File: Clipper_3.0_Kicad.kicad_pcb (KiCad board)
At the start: 2 copper layers, 19 parts, among them J10 Conn_01x19_Socket, J11 Screw_Terminal_01x02, J12 Conn_01x01_Socket, J13 Conn_01x01_Socket, J14 Conn_01x01_Socket, J15 Conn_01x01_Socket, J4 Conn_01x08_Socket, J5 Conn_01x08_Socket, J6 Conn_01x08_Socket, J9 Conn_01x19_Socket, U1 ESP32-DevKitC, U2 TB6612FNG_MODULE, U3 GY-521 MODULE, U4 DC/DC MINI-360

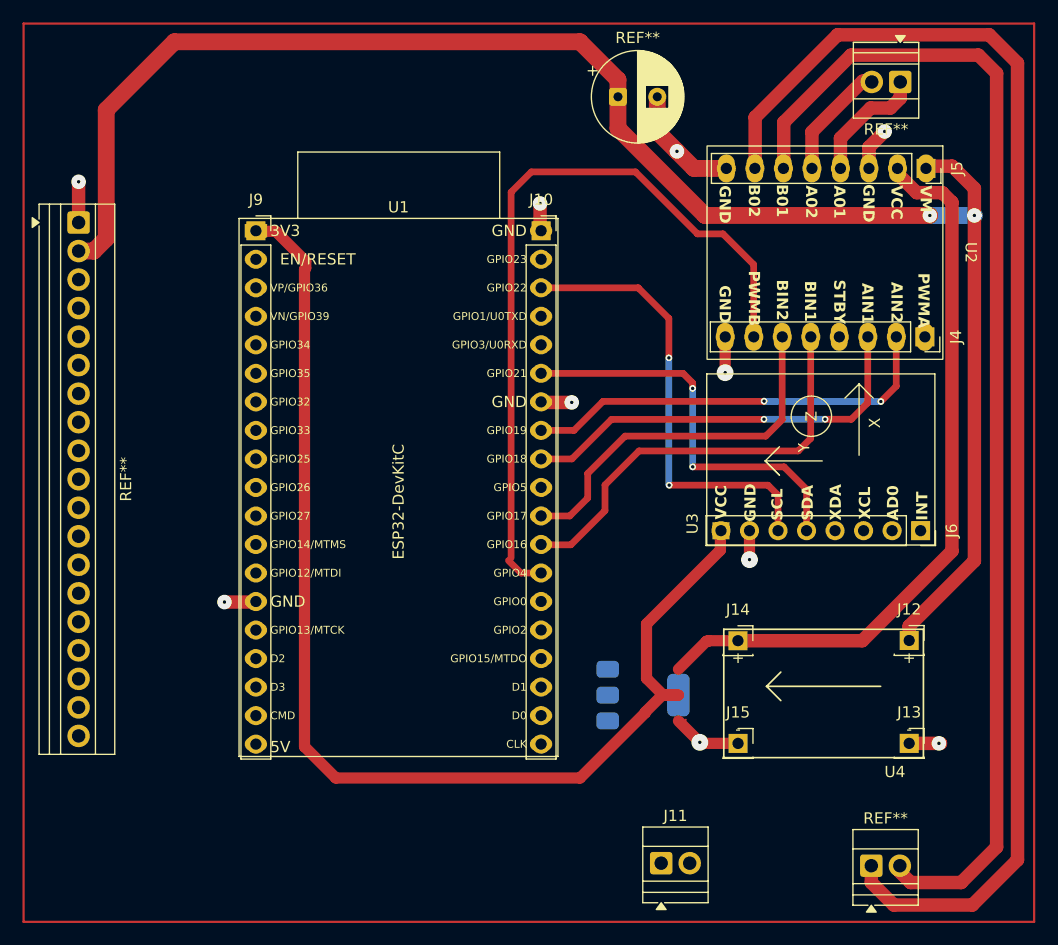
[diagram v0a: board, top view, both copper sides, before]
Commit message: Actualizacion de avance en SCH
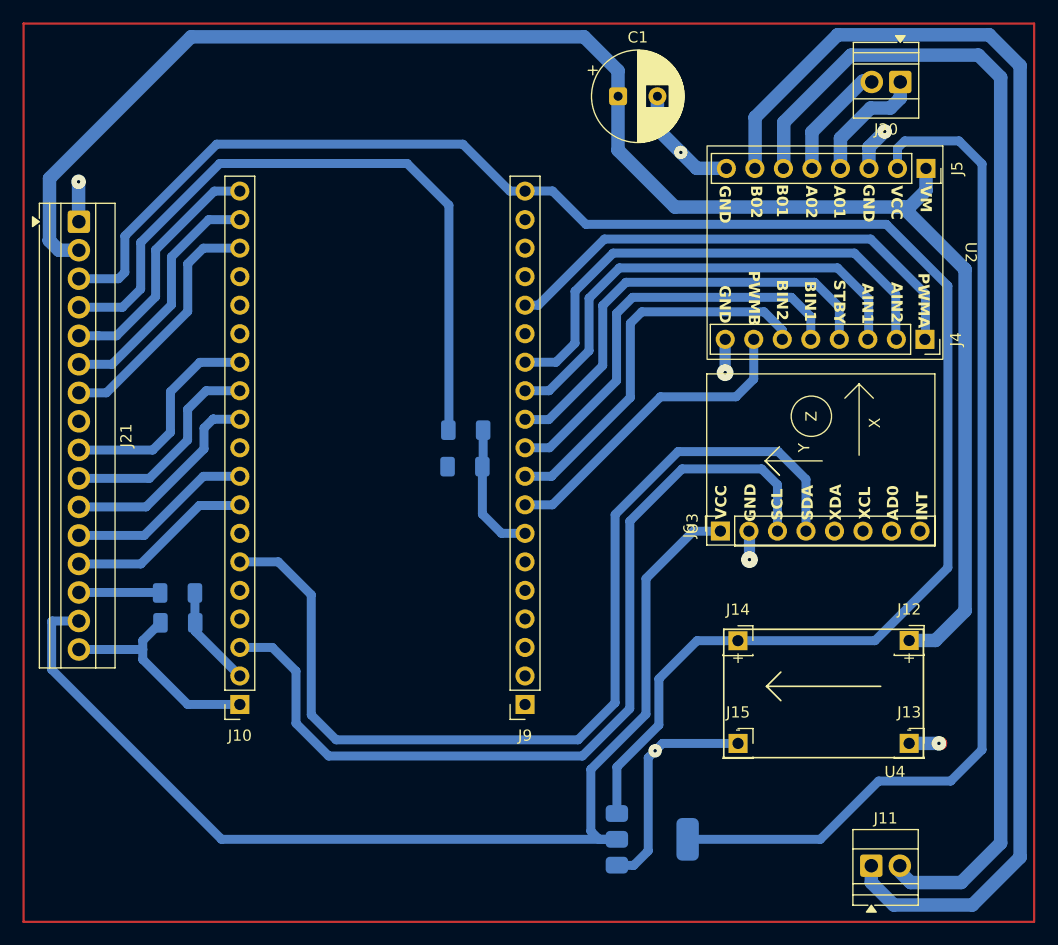
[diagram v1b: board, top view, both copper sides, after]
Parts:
- removed REF**: TerminalBlock_Xinya_XY308-2.54-19P_1x19_P2.54mm_Horizontal, TerminalBlock:TerminalBlock_Xinya_XY308-2.54-19P_1x19_P2.54mm_Horizontal
- removed REF**: CP_Radial_D8.0mm_P3.50mm, Capacitor_THT:CP_Radial_D8.0mm_P3.50mm
- removed REF** (x2): TerminalBlock_Xinya_XY308-2.54-2P_1x02_P2.54mm_Horizontal, TerminalBlock:TerminalBlock_Xinya_XY308-2.54-2P_1x02_P2.54mm_Horizontal
- removed REF**: SOT-223-3_TabPin2, Package_TO_SOT_SMD:SOT-223-3_TabPin2
- added C1: C_Polarized_Small, Capacitor_THT:CP_Radial_D8.0mm_P3.50mm, F.Cu at (161.4, 65.0)
- added J20: Screw_Terminal_01x02, TerminalBlock:TerminalBlock_Xinya_XY308-2.54-2P_1x02_P2.54mm_Horizontal, F.Cu at (186.6, 63.7)
- added J21: Screw_Terminal_01x16, TerminalBlock:TerminalBlock_Xinya_XY308-2.54-16P_1x16_P2.54mm_Horizontal, F.Cu at (113.4, 76.1)
- added R1: 3.3K, Resistor_SMD:R_1206_3216Metric_Pad1.30x1.75mm_HandSolder, B.Cu at (122.2, 109.2)
- added R2: 4.7K, Resistor_SMD:R_1206_3216Metric_Pad1.30x1.75mm_HandSolder, B.Cu at (122.2, 111.9)
- added R3: 3.3V, Resistor_SMD:R_1206_3216Metric_Pad1.30x1.75mm_HandSolder, B.Cu at (147.9, 94.7)
- added R4: 4.7K, Resistor_SMD:R_1206_3216Metric_Pad1.30x1.75mm_HandSolder, B.Cu at (147.8, 98.0)
- U5: renamed from U1; value ESP32-DevKitC -> AMS1117-3.3; footprint Espressif:ESP32-DevKitC -> Package_TO_SOT_SMD:SOT-223-3_TabPin2; moved to B.Cu
- moved U5 64.7 mm to (164.5, 131.2)
- moved J10 50.0 mm to (127.8, 119.1), turned to 180 degrees
- moved J9 48.5 mm to (153.2, 119.1), turned to 180 degrees
- moved J11 18.7 mm to (184.0, 133.5)
- moved J6 17.8 mm to (170.6, 103.7), turned to 90 degrees
- moved J4 0.22 mm to (188.8, 86.6)
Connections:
- J10 pad 1: unconnected-(J10-Pin_1-Pad1) -> GND
- J10 pad 11: unconnected-(J10-Pin_11-Pad11) -> S1
- J10 pad 12: unconnected-(J10-Pin_12-Pad12) -> S0
- J10 pad 13: unconnected-(J10-Pin_13-Pad13) -> SIG
- J10 pad 17: unconnected-(J10-Pin_17-Pad17) -> Net-(J10-Pin_17)
- J10 pad 18: unconnected-(J10-Pin_18-Pad18) -> /LED
- J10 pad 19: unconnected-(J10-Pin_19-Pad19) -> /BTN
- J10 pad 2: unconnected-(J10-Pin_2-Pad2) -> Net-(J10-Pin_2)
- J10 pad 3: unconnected-(J10-Pin_3-Pad3) -> Net-(J10-Pin_3)
- J10 pad 6: unconnected-(J10-Pin_6-Pad6) -> Net-(J10-Pin_6)
- J10 pad 7: unconnected-(J10-Pin_7-Pad7) -> GND
- J10 pad 8: unconnected-(J10-Pin_8-Pad8) -> S3
- J10 pad 9: unconnected-(J10-Pin_9-Pad9) -> S2
- J11 pad 1: unconnected-(J11-Pin_1-Pad1) -> /BO2
- J11 pad 2: unconnected-(J11-Pin_2-Pad2) -> /BO1
- J12 pad 1: unconnected-(J12-Pin_1-Pad1) -> VCC12V
- J13 pad 1: unconnected-(J13-Pin_1-Pad1) -> GND
- J14 pad 1: unconnected-(J14-Pin_1-Pad1) -> VCC5V
- J15 pad 1: unconnected-(J15-Pin_1-Pad1) -> GND
- J5 pad 1: /VM -> VCC12V
- J5 pad 2: /VCC -> VCC3.3V
- J6 pad 1: unconnected-(J6-Pin_1-Pad1) -> VCC3.3V
- J6 pad 2: unconnected-(J6-Pin_2-Pad2) -> GND
- J6 pad 3: unconnected-(J6-Pin_3-Pad3) -> Net-(J10-Pin_3)
- J6 pad 4: unconnected-(J6-Pin_4-Pad4) -> Net-(J10-Pin_6)
- J9 pad 10: unconnected-(J9-Pin_10-Pad10) -> /BIN1
- J9 pad 11: unconnected-(J9-Pin_11-Pad11) -> /STBY
- J9 pad 12: unconnected-(J9-Pin_12-Pad12) -> /AIN1
- J9 pad 13: unconnected-(J9-Pin_13-Pad13) -> /AIN2
- J9 pad 14: unconnected-(J9-Pin_14-Pad14) -> GND
- J9 pad 15: unconnected-(J9-Pin_15-Pad15) -> /PWMA
- J9 pad 19: unconnected-(J9-Pin_19-Pad19) -> VCC5V
- J9 pad 7: unconnected-(J9-Pin_7-Pad7) -> Net-(J9-Pin_7)
- J9 pad 8: unconnected-(J9-Pin_8-Pad8) -> /PWMB
- J9 pad 9: unconnected-(J9-Pin_9-Pad9) -> /BIN2
- U5 pad 1: unconnected-(U1-3V3-Pad1) -> GND
- U5 pad 2: unconnected-(U1-CHIP_PU-Pad2) -> VCC3.3V
- U5 pad 3: unconnected-(U1-SENSOR_VP/GPIO36/ADC1_CH0-Pad3) -> VCC5V
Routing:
- net VCC3.3V: track 0.00 -> 191.0 mm
- net VCC5V: track 0.00 -> 158.0 mm
- net unconnected-(U4-VCC_In-Pad1): track 151.1 -> 0.00 mm, vias 2 -> 0
- net VCC12V: track 0.00 -> 149.7 mm
- net /BO2: track 0.00 -> 120.2 mm
- net Net-(J2-Pin_7): track 120.0 -> 0.00 mm
- net Net-(J2-Pin_6): track 106.0 -> 0.00 mm
- net unconnected-(U3-VCC-Pad1): track 105.8 -> 0.00 mm
- net /BO1: track 0.00 -> 105.7 mm
- net Net-(J10-Pin_6): track 0.00 -> 89.3 mm
- net Net-(J10-Pin_3): track 0.00 -> 79.7 mm
- net Net-(J2-Pin_2): track 66.1 -> 0.00 mm
- net /ENCD: track 0.00 -> 62.3 mm
- net /PWMA: track 0.00 -> 44.2 mm
- net GND: track 22.5 -> 66.6 mm, vias 5 -> 7
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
